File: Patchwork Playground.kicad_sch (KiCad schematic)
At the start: 89 parts, among them J1 PADS, J2 USB_C_Receptacle_USB2.0, J3 PADS, J4 POGO, J5 PADS, J6 JST-GH-4P, SW1 SW_SPDT, SW2 SW_SPDT, SW3 SW_SPDT, SW4 BUTTON, SW5 SW_SPDT, SW6 SW_SPDT, SW7 SW_SPDT, U1 SMF05CT1G, U2 M3406, U3 BQ21040DBVR, U4 SMF05CT1G, U5 QMC5883L, U6 BC805M, U7 LSM6DSV

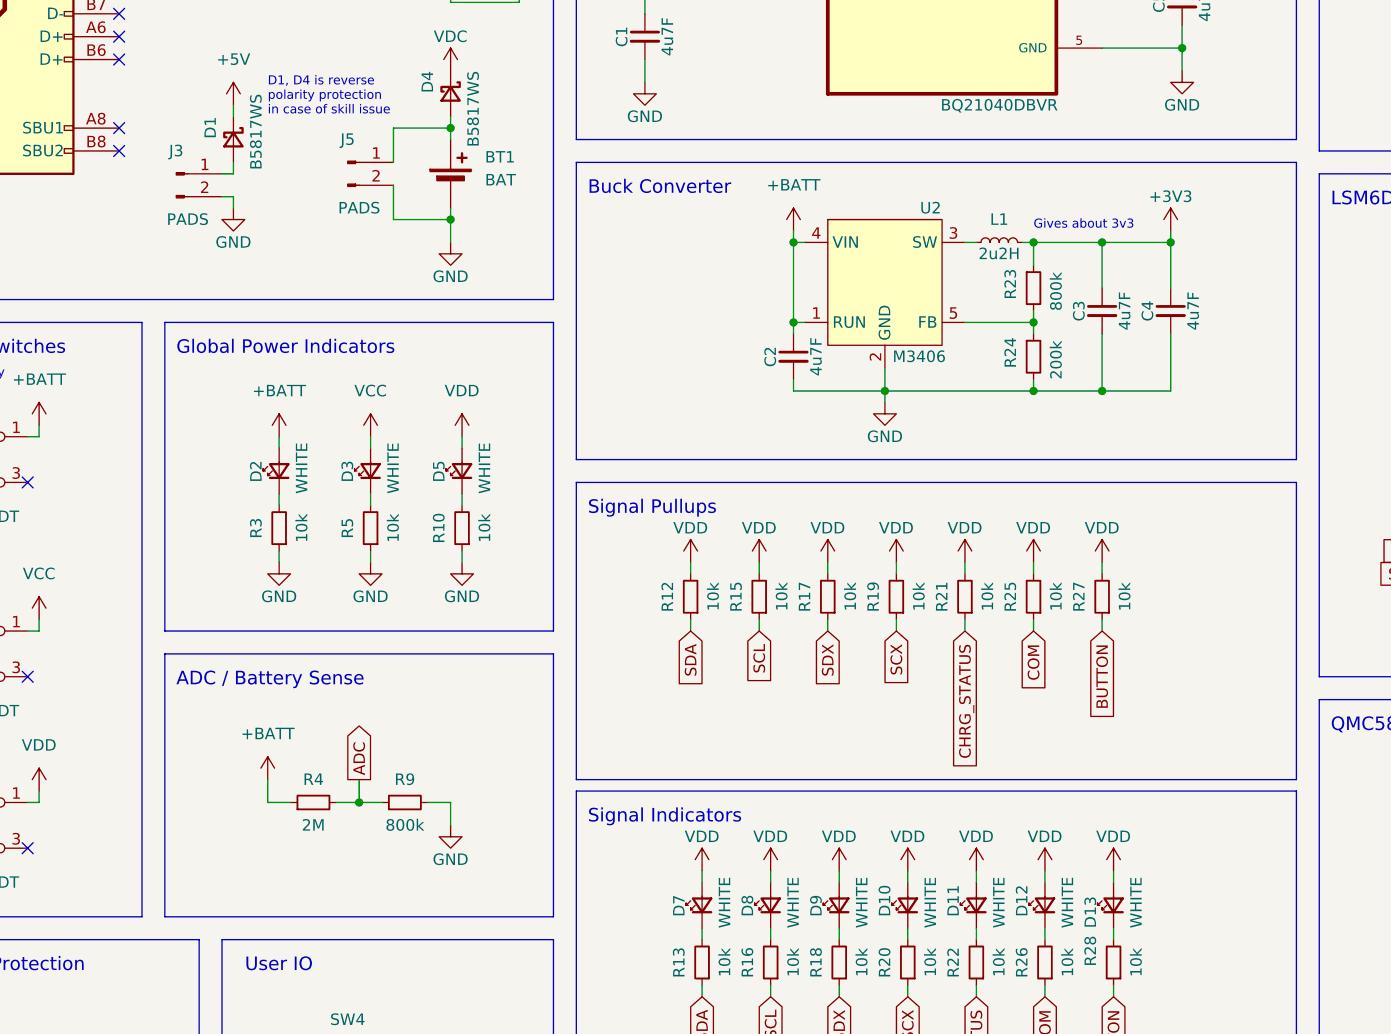
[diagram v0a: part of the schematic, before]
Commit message: Bom consolidation UwU
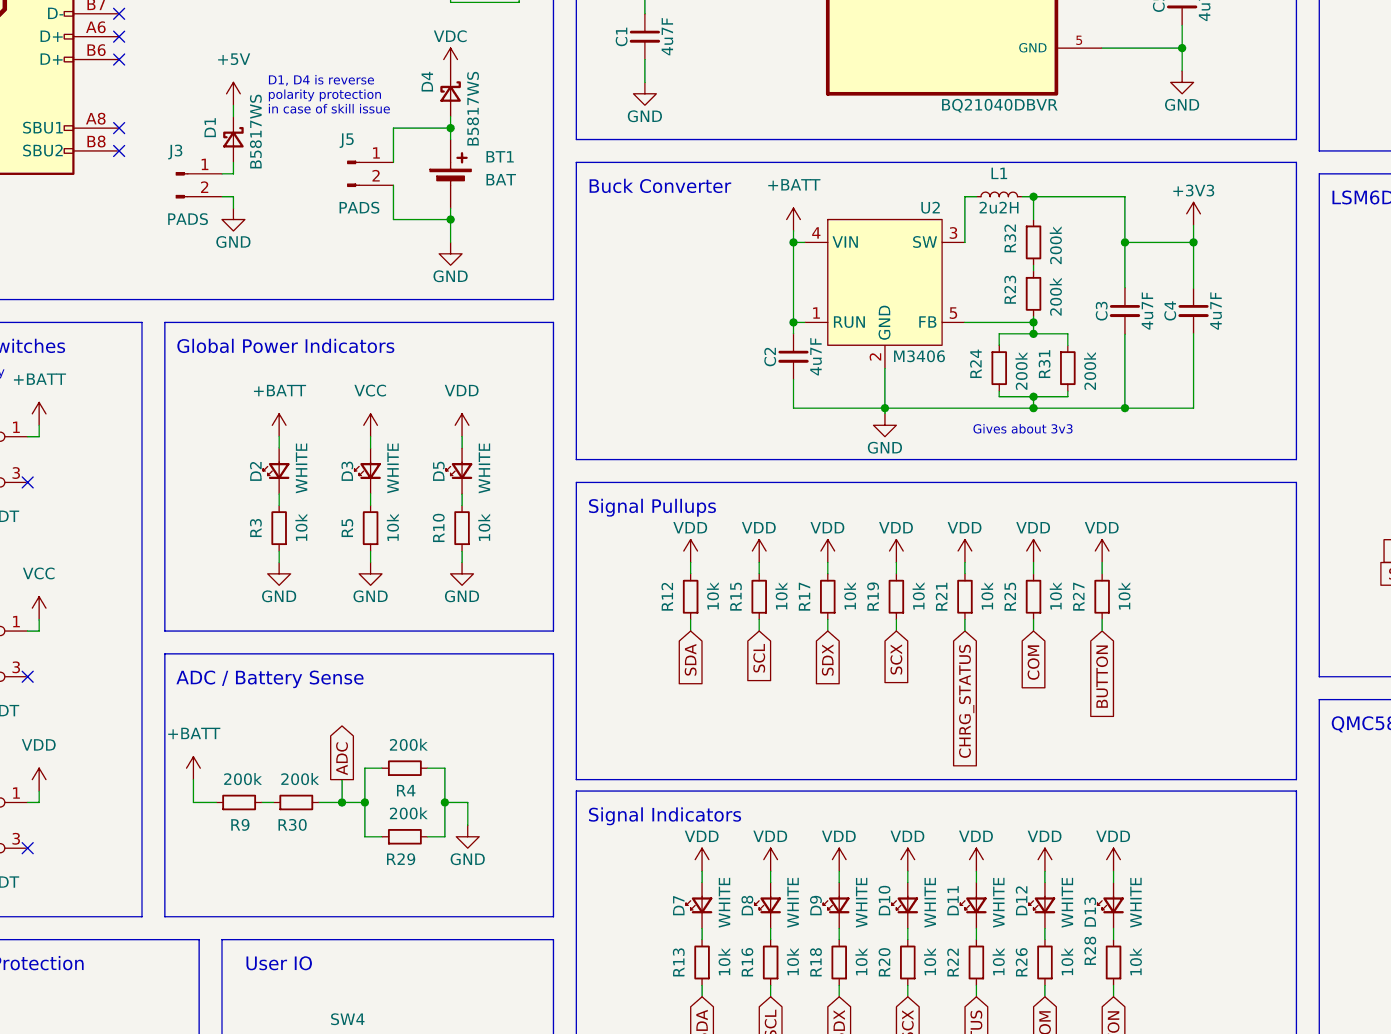
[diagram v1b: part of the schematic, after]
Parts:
- added R29, R30, R31, R32: 200k, Patchwork Playground Footprints:R_0603_1608Metric, symbol Patchwork Playground Symbols:R_Small
- BT1, J4, J6, U6: now left out of the parts list
- C1, C2, C3, C4, C5, C7: MPN (none) -> C19666
- C10, C6, C9: MPN (none) -> C14663
- C8: MPN (none) -> C21120
- D1, D4: EXTENDED? (none) -> YES; MPN (none) -> C5178966
- D10, D11, D12, D13, D2, D3, D5, D7, D8, D9: MPN (none) -> C2290
- D6: EXTENDED? (none) -> YES; MPN (none) -> C965844
- J2: MPN (none) -> C165948
- L1: EXTENDED? (none) -> YES; MPN (none) -> C285966
- R1, R2: MPN (none) -> C23186
- R10, R11, R12, R13, R14, R15, R16, R17, R18, R19, R20, R21, R22, R25, R26, R27, R28, R3, R5, R6, R7, R8: MPN (none) -> C25804
- R23, R9: value 800k -> 200k; MPN (none) -> C25811
- R24: MPN (none) -> C25811
- R4: value 2M -> 200k; MPN (none) -> C25811
- SW1, SW2, SW3, SW5, SW6, SW7: EXTENDED? (none) -> YES; MPN (none) -> C2875122
- SW4: MPN (none) -> C318884
- U1, U4: MPN (none) -> C15879
- U2: EXTENDED? (none) -> YES; MPN (none) -> C83224
- U3: EXTENDED? (none) -> YES; MPN (none) -> C202311
- U5: EXTENDED? (none) -> YES; MPN (none) -> C976032
- U7: EXTENDED? (none) -> YES; MPN (none) -> C9900037528
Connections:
- net +3V3: now also R32.1; no longer R23.1
- net +BATT: now also R9.1; no longer R4.1
- net ADC: now also R4.1, R29.1, R30.2; no longer R4.2, R9.1
- net GND: now also R4.2, R29.2, R31.2; no longer R9.2
- net at R23.2, R24.1, U2.5 (FB): now also R31.1
- new net: R30.1, R9.2
- new net: R23.1, R32.2
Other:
- moved on the sheet: C3, C4, L1, R24
